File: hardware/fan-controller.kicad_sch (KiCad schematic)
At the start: 29 parts, among them J1 DC_12V_IN, J2 HDD_POWER_OUT, J3 470531000, J4 470531000, Q1 2N3904, Q2 2N3904, U1 TSR0.5-2450, U2 XIAO-RP2350-SMD, U3 INA228

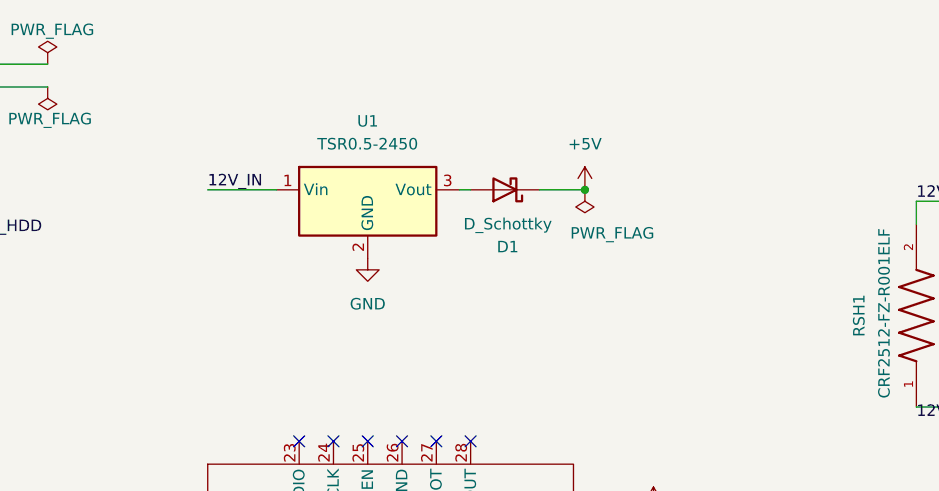
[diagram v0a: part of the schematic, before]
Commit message: run ERC
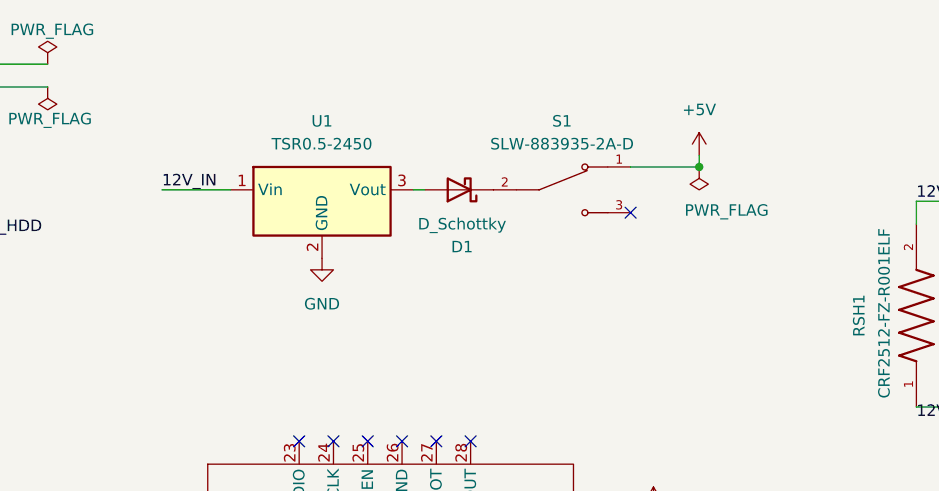
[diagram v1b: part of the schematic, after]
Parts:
- added S1: SLW-883935-2A-D, FanController:SW_SLW-883935-2A-D, symbol FanController:SLW-883935-2A-D
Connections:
- net +5V: now also S1.1; no longer D1.1 (K)
- new net: D1.1 (K), S1.2
- no-connect marks 21 -> 22
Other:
- moved on the sheet: D1, U1
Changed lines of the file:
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@@
 	(paper "A4")
 	(junction
-		(at 109.22 35.56)
-		(diameter 0)
-		(color 0 0 0 0)
-	)
-	(junction
 		(at 40.64 24.13)
 		(diameter 0)
@@
 	)
 	(junction
+		(at 121.92 33.02)
+		(diameter 0)
+		(color 0 0 0 0)
+	)
+	(junction
 		(at 198.12 33.02)
 		(diameter 0)
@@
 	)
 	(no_connect
+		(at 114.3 38.1)
+	)
+	(no_connect
 		(at 110.49 110.49)
 	)
@@
 	(wire
 		(pts
+			(xy 121.92 33.02) (xy 121.92 31.75)
+		)
+		(stroke
+			(width 0)
+			(type default)
+		)
+	)
+	(wire
+		(pts
 			(xy 110.49 86.36) (xy 116.84 86.36)
 		)
@@
 	(wire
 		(pts
-			(xy 95.25 35.56) (xy 96.52 35.56)
+			(xy 90.17 35.56) (xy 91.44 35.56)
 		)
 		(stroke
@@
 	(wire
 		(pts
-			(xy 104.14 35.56) (xy 109.22 35.56)
-		)
-		(stroke
-			(width 0)
-			(type default)
-		)
-	)
-	(wire
-		(pts
 			(xy 99.06 163.83) (xy 109.22 163.83)
 		)
@@
 	(wire
 		(pts
-			(xy 67.31 35.56) (xy 74.93 35.56)
+			(xy 62.23 35.56) (xy 69.85 35.56)
 		)
 		(stroke
@@
 	(wire
 		(pts
+			(xy 114.3 33.02) (xy 121.92 33.02)
+		)
+		(stroke
+			(width 0)
+			(type default)
+		)
+	)
+	(wire
+		(pts
 			(xy 208.28 49.53) (xy 210.82 49.53)
 		)
@@
 	)
 	(label "12V_IN"
-		(at 67.31 35.56 0)
+		(at 62.23 35.56 0)
 		(effects
 			(font
@@
 	)
 	(symbol
+		(lib_id "FanController:SLW-883935-2A-D")
+		(at 106.68 35.56 0)
+		(unit 1)
+		(body_style 1)
+		(exclude_from_sim no)
+		(in_bom yes)
+		(on_board yes)
+		(in_pos_files yes)
+		(dnp no)
+		(fields_autoplaced yes)
+		(property "Reference" "S1"
+			(at 106.68 27.94 0)
+			(show_name no)
+			(do_not_autoplace no)
+			(effects
+				(font
+					(size 1.27 1.27)
+				)
+			)
+		)
+		(property "Value" "SLW-883935-2A-D"
+			(at 106.68 30.48 0)
+			(show_name no)
+			(do_not_autoplace no)
+			(effects
+				(font
+					(size 1.27 1.27)
+				)
+			)
+		)
+		(property "Footprint" "FanController:SW_SLW-883935-2A-D"
+			(at 106.68 35.56 0)
+			(hide yes)
+			(show_name no)
+			(do_not_autoplace no)
+			(effects
+				(font
+					(size 1.27 1.27)
+				)
+				(justify bottom)
+			)
+		)
+		(property "Datasheet" ""
+			(at 106.68 35.56 0)
+			(hide yes)
+			(show_name no)
+			(do_not_autoplace no)
+			(effects
+				(font
+					(size 1.27 1.27)
+				)
+			)
+		)
+		(property "Description" ""
+			(at 106.68 35.56 0)
+			(hide yes)
+			(show_name no)
+			(do_not_autoplace no)
+			(effects
+				(font
+					(size 1.27 1.27)
+				)
+			)
+		)
+		(property "PARTREV" "1.01"
+			(at 106.68 35.56 0)
+			(hide yes)
+			(show_name no)
+			(do_not_autoplace no)
+			(effects
+				(font
+					(size 1.27 1.27)
+				)
+				(justify bottom)
+			)
+		)
+		(property "STANDARD" "Manufacturer Recommendations"
+			(at 106.68 35.56 0)
+			(hide yes)
+			(show_name no)
+			(do_not_autoplace no)
+			(effects
+				(font
+					(size 1.27 1.27)
+				)
+				(justify bottom)
+			)
+		)
+		(property "MAXIMUM_PACKAGE_HEIGHT" "6.1mm"
+			(at 106.68 35.56 0)
+			(hide yes)
+			(show_name no)
+			(do_not_autoplace no)
+			(effects
+				(font
+					(size 1.27 1.27)
+				)
+				(justify bottom)
+			)
+		)
+		(property "MANUFACTURER" "Same Sky"
+			(at 106.68 35.56 0)
+			(hide yes)
+			(show_name no)
+			(do_not_autoplace no)
+			(effects
+				(font
+					(size 1.27 1.27)
+				)
+				(justify bottom)
+			)
+		)
+		(pin "1"
+		)
+		(pin "2"
+		)
+		(pin "3"
+		)
+		(instances
+			(project "fan-controller"
+				(path "/2efa048c-d6c1-446c-ae8e-880d974401eb"
+					(reference "S1")
+					(unit 1)
+				)
+			)
+		)
+	)
+	(symbol
 		(lib_id "power:PWR_FLAG")
 		(at 49.53 21.59 0)
@@
 	(symbol
 		(lib_id "power:PWR_FLAG")
-		(at 109.22 35.56 0)
+		(at 121.92 33.02 0)
 		(mirror x)
 		(unit 1)
@@
 		(dnp no)
 		(property "Reference" "#FLG03"
-			(at 109.22 37.465 0)
+			(at 121.92 34.925 0)
 			(hide yes)
 			(show_name no)
@@
 		)
 		(property "Value" "PWR_FLAG"
-			(at 112.268 40.386 0)
+			(at 124.968 37.846 0)
 			(show_name no)
 			(do_not_autoplace no)
@@
 		)
 		(property "Footprint" ""
-			(at 109.22 35.56 0)
+			(at 121.92 33.02 0)
 			(hide yes)
 			(show_name no)
@@
 		)
 		(property "Datasheet" ""
-			(at 109.22 35.56 0)
+			(at 121.92 33.02 0)
 			(hide yes)
 			(show_name no)
@@
 		)
 		(property "Description" "Special symbol for telling ERC where power comes from"
-			(at 109.22 35.56 0)
+			(at 121.92 33.02 0)
 			(hide yes)
 			(show_name no)
@@
 	(symbol
 		(lib_id "power:+5V")
-		(at 109.22 35.56 0)
+		(at 121.92 31.75 0)
 		(unit 1)
 		(body_style 1)
@@
 		(fields_autoplaced yes)
 		(property "Reference" "#PWR09"
-			(at 109.22 39.37 0)
+			(at 121.92 35.56 0)
 			(hide yes)
 			(show_name no)
@@
 		)
 		(property "Value" "+5V"
-			(at 109.22 30.48 0)
+			(at 121.92 26.67 0)
 			(show_name no)
 			(do_not_autoplace no)
@@
 		)
 		(property "Footprint" ""
-			(at 109.22 35.56 0)
+			(at 121.92 31.75 0)
 			(hide yes)
 			(show_name no)
@@
 		)
 		(property "Datasheet" ""
-			(at 109.22 35.56 0)
+			(at 121.92 31.75 0)
 			(hide yes)
 			(show_name no)
@@
 		)
 		(property "Description" "Power symbol creates a global label with name \"+5V\""
-			(at 109.22 35.56 0)
+			(at 121.92 31.75 0)
 			(hide yes)
 			(show_name no)
@@
 	(symbol
 		(lib_id "power:GND")
-		(at 85.09 43.18 0)
+		(at 80.01 43.18 0)
 		(unit 1)
 		(body_style 1)
@@
 		(fields_autoplaced yes)
 		(property "Reference" "#PWR05"
-			(at 85.09 49.53 0)
+			(at 80.01 49.53 0)
 			(hide yes)
 			(show_name no)
@@
 		)
 		(property "Value" "GND"
-			(at 85.09 48.26 0)
+			(at 80.01 48.26 0)
 			(show_name no)
 			(do_not_autoplace no)
@@
 		)
 		(property "Footprint" ""
-			(at 85.09 43.18 0)
+			(at 80.01 43.18 0)
 			(hide yes)
 			(show_name no)
@@
 		)
 		(property "Datasheet" ""
-			(at 85.09 43.18 0)
+			(at 80.01 43.18 0)
 			(hide yes)
 			(show_name no)
@@
 		)
 		(property "Description" "Power symbol creates a global label with name \"GND\" , ground"
-			(at 85.09 43.18 0)
+			(at 80.01 43.18 0)
 			(hide yes)
 			(show_name no)
@@
 	(symbol
 		(lib_id "Device:D_Schottky")
-		(at 100.33 35.56 180)
+		(at 95.25 35.56 180)
 		(unit 1)
 		(body_style 1)
@@
 		(fields_autoplaced yes)
 		(property "Reference" "D1"
-			(at 100.6475 41.91 0)
+			(at 95.5675 41.91 0)
 			(show_name no)
 			(do_not_autoplace no)
@@
 		)
 		(property "Value" "D_Schottky"
-			(at 100.6475 39.37 0)
+			(at 95.5675 39.37 0)
 			(show_name no)
 			(do_not_autoplace no)
@@
 		)
 		(property "Footprint" "Diode_SMD:D_SOD-123F"
-			(at 100.33 35.56 0)
+			(at 95.25 35.56 0)
 			(hide yes)
 			(show_name no)
@@
 		)
 		(property "Datasheet" "https://www.st.com/resource/en/datasheet/stps1l40.pdf"
-			(at 100.33 35.56 0)
+			(at 95.25 35.56 0)
 			(hide yes)
 			(show_name no)
@@
 		)
 		(property "Description" "STPS1L40ZF"
-			(at 100.33 35.56 0)
+			(at 95.25 35.56 0)
 			(hide yes)
 			(show_name no)
@@
 	(symbol
 		(lib_id "Converter_DCDC:TSR0.5-2450")
-		(at 85.09 38.1 0)
+		(at 80.01 38.1 0)
 		(unit 1)
 		(body_style 1)
@@
 		(fields_autoplaced yes)
 		(property "Reference" "U1"
-			(at 85.09 27.94 0)
+			(at 80.01 27.94 0)
 			(show_name no)
 			(do_not_autoplace no)
@@
 		)
 		(property "Value" "TSR0.5-2450"
-			(at 85.09 30.48 0)
+			(at 80.01 30.48 0)
 			(show_name no)
 			(do_not_autoplace no)
@@
 		)
 		(property "Footprint" "Converter_DCDC:Converter_DCDC_TRACO_TSR0.5-24xx_TSR0.5-24xxx_THT"
-			(at 85.09 44.196 0)
+			(at 80.01 44.196 0)
 			(hide yes)
 			(show_name no)
@@
 		)
 		(property "Datasheet" "https://www.tracopower.com/products/tsr0.5.pdf"
-			(at 85.09 41.91 0)
+			(at 80.01 41.91 0)
 			(hide yes)
 			(show_name no)
@@
 		)
 		(property "Description" "0.5A step-down regulator, fixed 5V output voltage, 6.5-32V input voltage, TO-220 compatible LM78xx replacement, SIP-3"
-			(at 85.09 38.1 0)
+			(at 80.01 38.1 0)
 			(hide yes)
 			(show_name no)
